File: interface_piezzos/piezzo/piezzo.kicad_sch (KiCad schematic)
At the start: 16 parts, among them J101 2350514-4, U101 TLV9302IDR

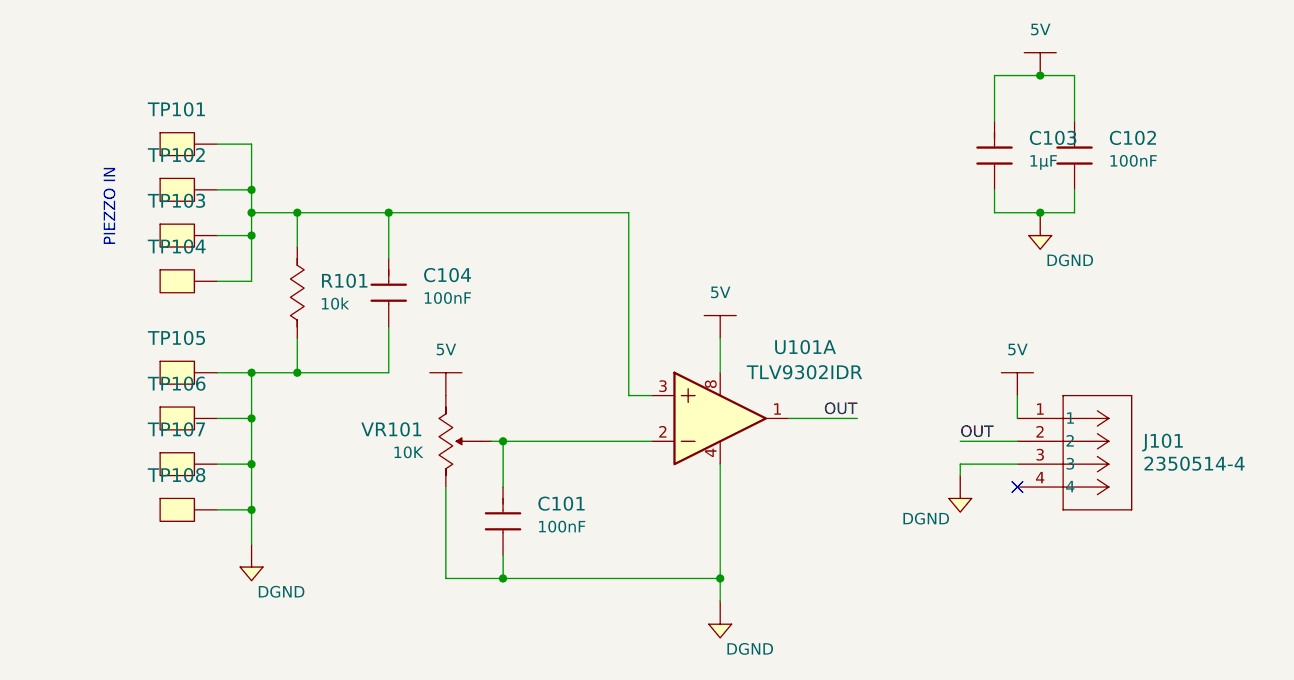
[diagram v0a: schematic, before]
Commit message: gerber + commande JLC
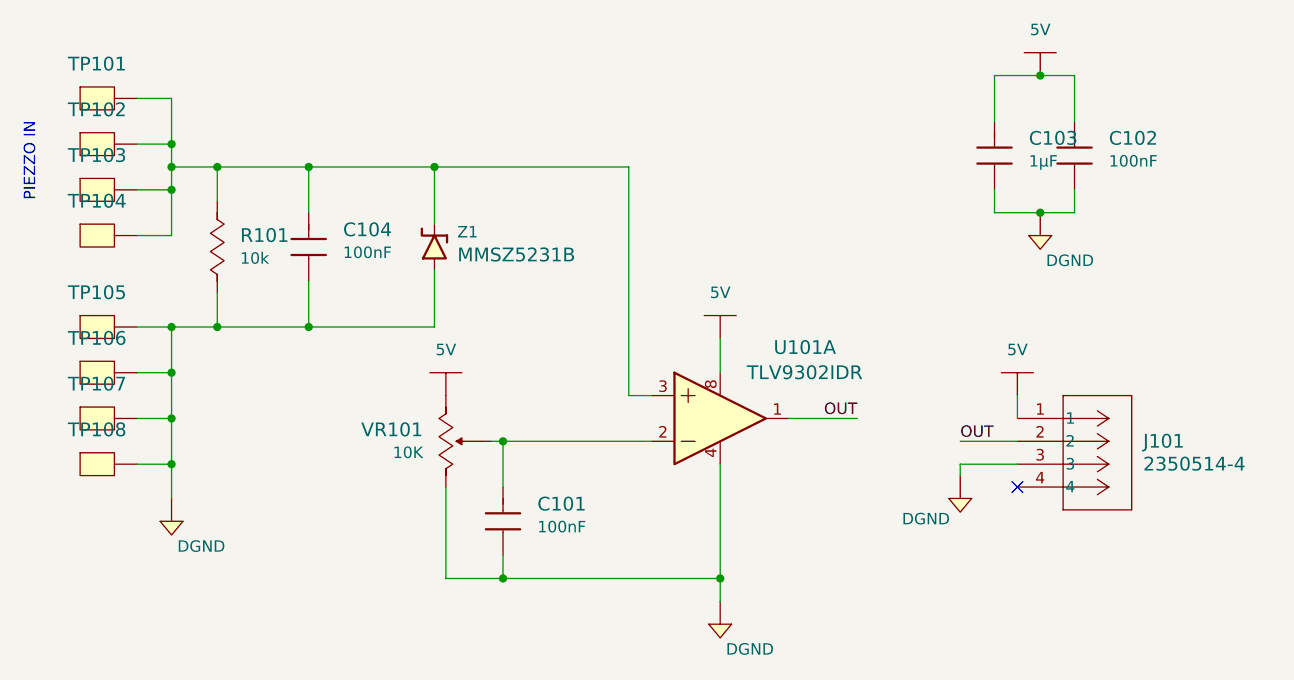
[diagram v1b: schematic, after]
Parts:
- added Z1: MMSZ5231B, Diodes:SOD-123FL, symbol Diodes:MMSZ5231B-7-F
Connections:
- net DGND: now also Z1.2 (Anode)
- net at C104.2, R101.2, TP101.1 (TP)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: now also Z1.1 (Cathode)
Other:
- moved on the sheet: C104, R101, TP101, TP102, TP103, TP104, TP105, TP106, TP107, TP108
